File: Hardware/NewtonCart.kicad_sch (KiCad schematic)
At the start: 17 parts, among them J1 Battery Pins, J2 TP4056 Module, J3 Reserve IO's, J4 UART2TTL Bridge, J5 BoostConverter, J6 MPU6050, J7 HX711, J8 HC-SR04, J9 FOTOELECTRIC_ENCODER, U1 ESP32-WROOM-32, U2 LM1117-3.3

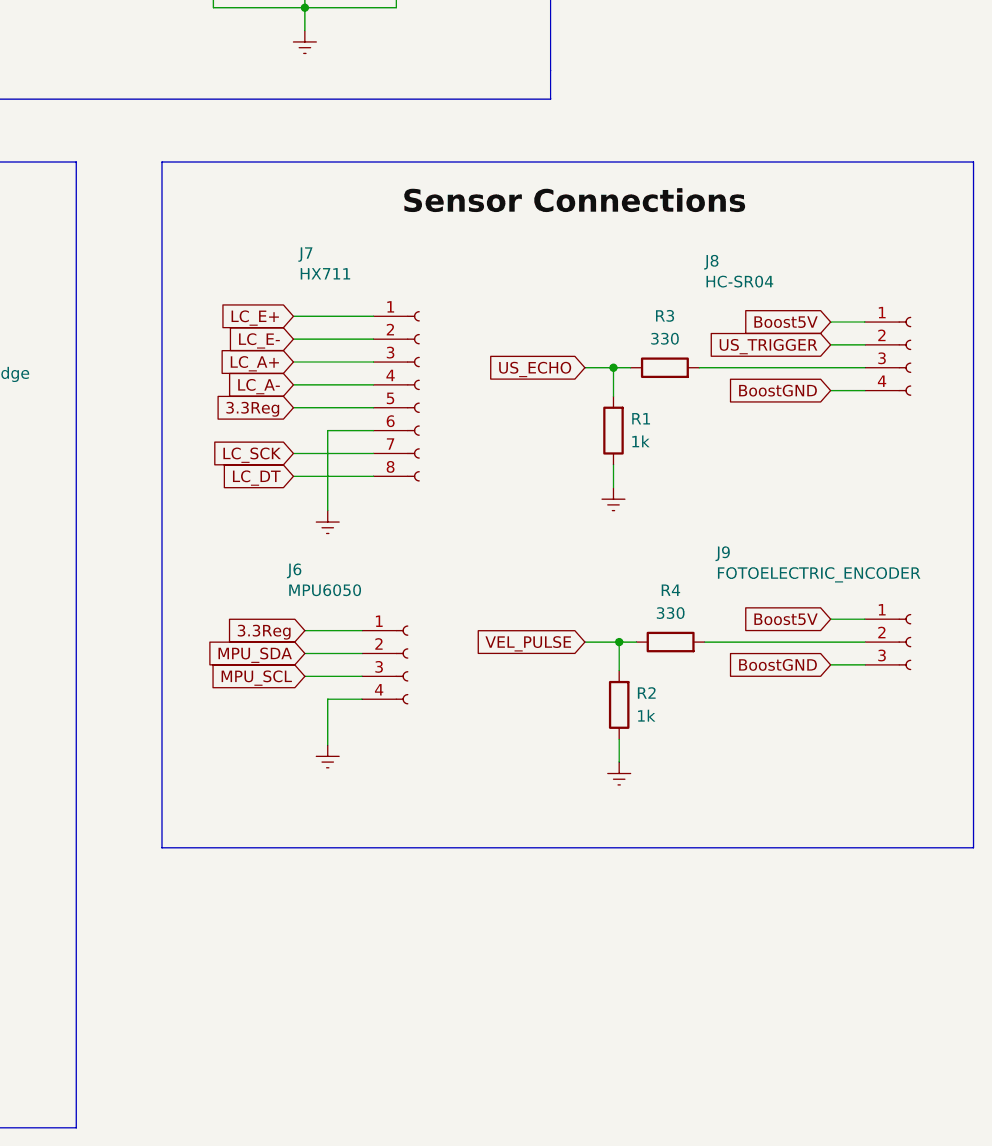
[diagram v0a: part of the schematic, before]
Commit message: Created Netlist, Locating PCB Boart components. Some schematic changes.
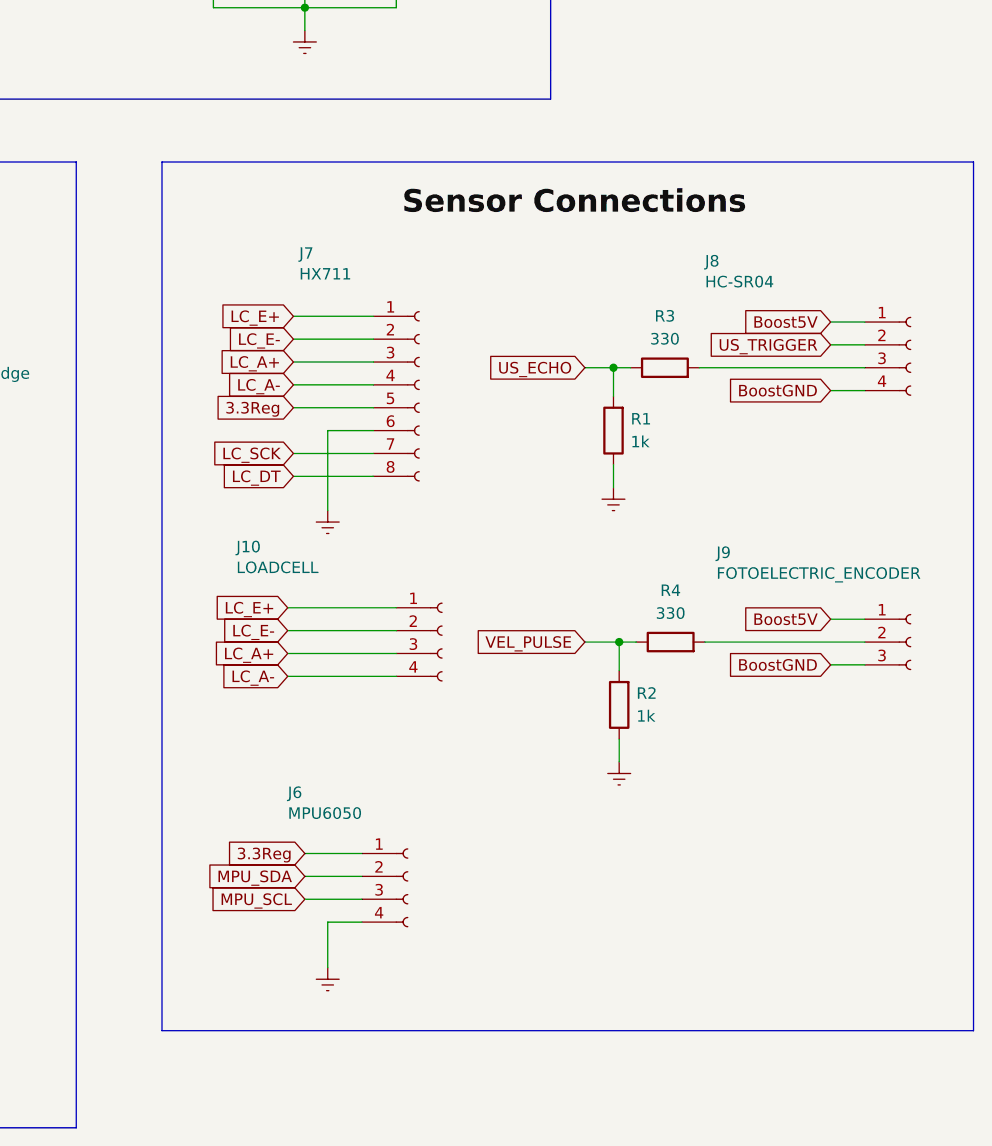
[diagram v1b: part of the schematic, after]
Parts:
- added J10: LOADCELL, Connector_PinHeader_2.54mm:PinHeader_1x04_P2.54mm_Vertical, symbol Connector:Conn_01x04_Female
- C1, C2: footprint (none) -> Resistor_THT:R_Axial_DIN0204_L3.6mm_D1.6mm_P5.08mm_Horizontal
- J1, J8: footprint (none) -> Connector_PinHeader_2.54mm:PinHeader_1x04_P2.54mm_Vertical
- J2: footprint (none) -> Miscelaneos:18650 TP4056 Module
- J3, J9: footprint (none) -> Connector_PinHeader_2.54mm:PinHeader_1x03_P2.54mm_Vertical
- J4: footprint (none) -> Connector_PinHeader_2.54mm:PinHeader_1x05_P2.54mm_Vertical
- J5: footprint (none) -> Miscelaneos:5-12V BoostConverter
- J6: footprint (none) -> Miscelaneos:MPU 6050 Module
- J7: footprint (none) -> Miscelaneos:HX711 Loadcell ADC
- R1, R2, R3, R4: footprint (none) -> Resistor_THT:R_Axial_DIN0309_L9.0mm_D3.2mm_P12.70mm_Horizontal
- U2: footprint (none) -> Package_TO_SOT_THT:TO-220-3_Vertical
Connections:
- net LC_A+: now also J10.3 (Pin_3)
- net LC_A-: now also J10.4 (Pin_4)
- net LC_E+: now also J10.1 (Pin_1)
- net LC_E-: now also J10.2 (Pin_2)
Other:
- moved on the sheet: J6

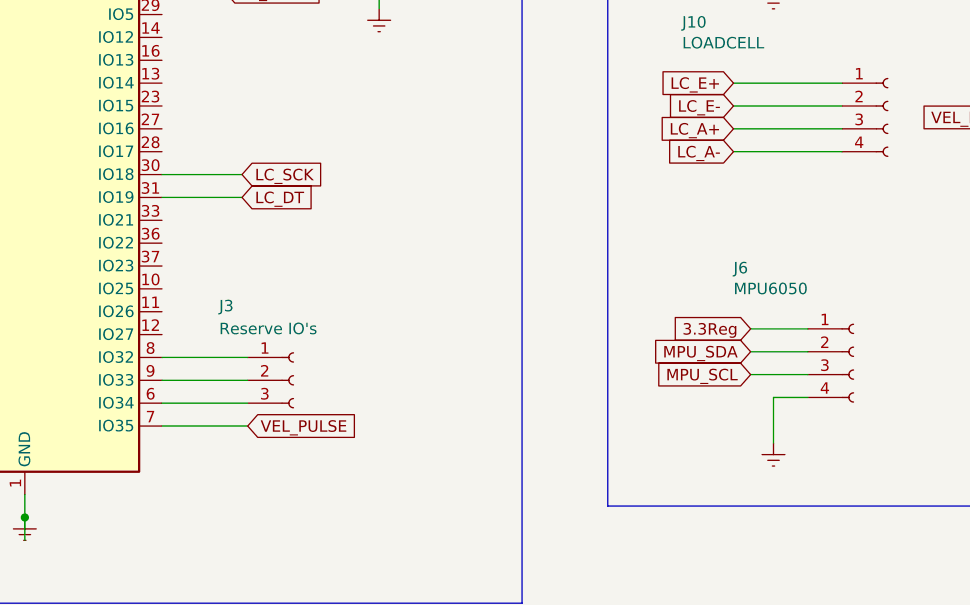
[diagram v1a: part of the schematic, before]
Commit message: Cambios Placa al 190322
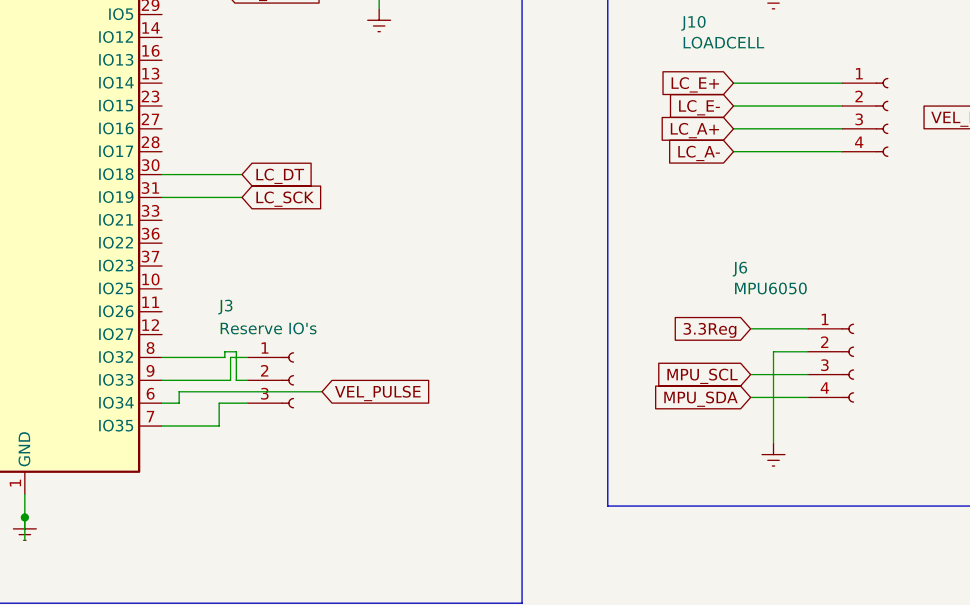
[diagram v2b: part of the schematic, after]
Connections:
- net Earth: now also J6.2 (Pin_2); no longer J6.4 (Pin_4)
- net LC_DT: now also U1.30 (IO18); no longer U1.31 (IO19)
- net LC_SCK: now also U1.31 (IO19); no longer U1.30 (IO18)
- net MPU_SDA: now also J6.4 (Pin_4); no longer J6.2 (Pin_2)
- net VEL_PULSE: now also U1.6 (IO34); no longer U1.7 (IO35)
- net at J3.3 (Pin_3): now also U1.7 (IO35); no longer U1.6 (IO34)
- net at U1.8 (IO32): now also J3.2 (Pin_2); no longer J3.1 (Pin_1)
- net at U1.9 (IO33): now also J3.1 (Pin_1); no longer J3.2 (Pin_2)
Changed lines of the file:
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@@
+    (stroke (width 0) (type default) (color 0 0 0 0))
+  )
+  (wire (pts (xy 145.415 147.955) (xy 151.765 147.955))
     (stroke (width 0) (type default) (color 0 0 0 0))
   )
@@
     (stroke (width 0) (type default) (color 0 0 0 0))
   )
+  (wire (pts (xy 147.955 145.415) (xy 147.955 155.575))
+    (stroke (width 0) (type default) (color 0 0 0 0))
+  )
   (wire (pts (xy 105.41 92.71) (xy 91.44 92.71))
     (stroke (width 0) (type default) (color 0 0 0 0))
   )
-  (wire (pts (xy 151.765 150.495) (xy 147.955 150.495))
-    (stroke (width 0) (type default) (color 0 0 0 0))
-  )
   (wire (pts (xy 203.835 116.84) (xy 207.645 116.84))
     (stroke (width 0) (type default) (color 0 0 0 0))
@@
     (stroke (width 0) (type default) (color 0 0 0 0))
   )
+  (wire (pts (xy 80.01 128.27) (xy 88.9 128.27))
+    (stroke (width 0) (type default) (color 0 0 0 0))
+  )
   (polyline (pts (xy 19.685 59.055) (xy 19.685 16.51))
     (stroke (width 0) (type default) (color 0 0 0 0))
@@
     (stroke (width 0) (type default) (color 0 0 0 0))
   )
-  (wire (pts (xy 80.01 148.59) (xy 89.535 148.59))
+  (wire (pts (xy 89.535 146.05) (xy 87.63 146.05))
+    (stroke (width 0) (type default) (color 0 0 0 0))
+  )
+  (wire (pts (xy 97.79 149.86) (xy 81.915 149.86))
     (stroke (width 0) (type default) (color 0 0 0 0))
   )
@@
     (stroke (width 0) (type default) (color 0 0 0 0))
   )
+  (wire (pts (xy 88.265 145.415) (xy 86.995 145.415))
+    (stroke (width 0) (type default) (color 0 0 0 0))
+  )
+  (wire (pts (xy 80.01 125.73) (xy 88.9 125.73))
+    (stroke (width 0) (type default) (color 0 0 0 0))
+  )
   (wire (pts (xy 101.6 100.33) (xy 101.6 102.87))
     (stroke (width 0) (type default) (color 0 0 0 0))
@@
     (stroke (width 0) (type default) (color 0 0 0 0))
   )
-  (wire (pts (xy 80.01 151.13) (xy 89.535 151.13))
+  (wire (pts (xy 81.915 151.13) (xy 80.01 151.13))
+    (stroke (width 0) (type default) (color 0 0 0 0))
+  )
+  (wire (pts (xy 87.63 148.59) (xy 80.01 148.59))
     (stroke (width 0) (type default) (color 0 0 0 0))
   )
@@
     (stroke (width 0) (type default) (color 0 0 0 0))
   )
-  (wire (pts (xy 80.01 125.73) (xy 88.9 125.73))
+  (wire (pts (xy 88.265 148.59) (xy 88.265 145.415))
     (stroke (width 0) (type default) (color 0 0 0 0))
   )
@@
     (stroke (width 0) (type default) (color 0 0 0 0))
   )
-  (wire (pts (xy 80.01 146.05) (xy 89.535 146.05))
-    (stroke (width 0) (type default) (color 0 0 0 0))
-  )
   (wire (pts (xy 73.66 41.275) (xy 77.47 41.275))
     (stroke (width 0) (type default) (color 0 0 0 0))
@@
     (stroke (width 0) (type default) (color 0 0 0 0))
   )
+  (wire (pts (xy 147.955 145.415) (xy 151.765 145.415))
+    (stroke (width 0) (type default) (color 0 0 0 0))
+  )
+  (wire (pts (xy 86.995 145.415) (xy 86.995 146.05))
+    (stroke (width 0) (type default) (color 0 0 0 0))
+  )
   (wire (pts (xy 91.44 80.645) (xy 94.615 80.645))
     (stroke (width 0) (type default) (color 0 0 0 0))
@@
     (stroke (width 0) (type default) (color 0 0 0 0))
   )
-  (wire (pts (xy 147.955 150.495) (xy 147.955 155.575))
-    (stroke (width 0) (type default) (color 0 0 0 0))
-  )
   (wire (pts (xy 35.56 46.99) (xy 39.37 46.99))
     (stroke (width 0) (type default) (color 0 0 0 0))
@@
     (stroke (width 0) (type default) (color 0 0 0 0))
   )
+  (wire (pts (xy 86.995 146.05) (xy 80.01 146.05))
+    (stroke (width 0) (type default) (color 0 0 0 0))
+  )
+  (wire (pts (xy 86.36 153.67) (xy 80.01 153.67))
+    (stroke (width 0) (type default) (color 0 0 0 0))
+  )
+  (wire (pts (xy 145.415 150.495) (xy 151.765 150.495))
+    (stroke (width 0) (type default) (color 0 0 0 0))
+  )
   (wire (pts (xy 143.51 120.65) (xy 155.575 120.65))
     (stroke (width 0) (type default) (color 0 0 0 0))
@@
     (stroke (width 0) (type default) (color 0 0 0 0))
   )
-  (wire (pts (xy 151.765 145.415) (xy 145.415 145.415))
-    (stroke (width 0) (type default) (color 0 0 0 0))
-  )
   (wire (pts (xy 203.835 83.82) (xy 207.645 83.82))
     (stroke (width 0) (type default) (color 0 0 0 0))
@@
     (stroke (width 0) (type default) (color 0 0 0 0))
   )
+  (wire (pts (xy 89.535 151.13) (xy 86.36 151.13))
+    (stroke (width 0) (type default) (color 0 0 0 0))
+  )
   (wire (pts (xy 129.54 37.465) (xy 135.255 37.465))
     (stroke (width 0) (type default) (color 0 0 0 0))
@@
     (stroke (width 0) (type default) (color 0 0 0 0))
   )
+  (wire (pts (xy 86.36 151.13) (xy 86.36 153.67))
+    (stroke (width 0) (type default) (color 0 0 0 0))
+  )
   (wire (pts (xy 203.835 121.92) (xy 207.645 121.92))
     (stroke (width 0) (type default) (color 0 0 0 0))
@@
     (stroke (width 0) (type default) (color 0 0 0 0))
   )
-  (wire (pts (xy 151.765 147.955) (xy 145.415 147.955))
-    (stroke (width 0) (type default) (color 0 0 0 0))
-  )
   (polyline (pts (xy 19.685 16.51) (xy 172.72 16.51))
     (stroke (width 0) (type default) (color 0 0 0 0))
   )
-  (wire (pts (xy 80.01 128.27) (xy 88.9 128.27))
+  (wire (pts (xy 81.915 149.86) (xy 81.915 151.13))
     (stroke (width 0) (type default) (color 0 0 0 0))
   )
@@
     (stroke (width 0) (type default) (color 0 0 0 0))
   )
+  (wire (pts (xy 89.535 148.59) (xy 88.265 148.59))
+    (stroke (width 0) (type default) (color 0 0 0 0))
+  )
   (wire (pts (xy 101.6 102.87) (xy 80.01 102.87))
     (stroke (width 0) (type default) (color 0 0 0 0))
@@
     (stroke (width 0) (type default) (color 0 0 0 0))
   )
+  (wire (pts (xy 87.63 146.05) (xy 87.63 148.59))
+    (stroke (width 0) (type default) (color 0 0 0 0))
+  )
   (wire (pts (xy 29.21 39.37) (xy 35.56 39.37))
-    (stroke (width 0) (type default) (color 0 0 0 0))
-  )
-  (wire (pts (xy 80.01 153.67) (xy 89.535 153.67))
     (stroke (width 0) (type default) (color 0 0 0 0))
   )
@@
     )
   )
-  (global_label "VEL_PULSE" (shape input) (at 89.535 153.67 0) (fields_autoplaced)
-    (effects (font (size 1.27 1.27)) (justify left))
-    (property "Intersheet References" "${INTERSHEET_REFS}" (id 0) (at 102.0797 153.5906 0)
+  (global_label "VEL_PULSE" (shape input) (at 97.79 149.86 0) (fields_autoplaced)
+    (effects (font (size 1.27 1.27)) (justify left))
+    (property "Intersheet References" "${INTERSHEET_REFS}" (id 0) (at 110.3347 149.7806 0)
       (effects (font (size 1.27 1.27)) (justify left) hide)
     )
@@
     )
   )
-  (global_label "LC_DT" (shape input) (at 88.9 128.27 0) (fields_autoplaced)
-    (effects (font (size 1.27 1.27)) (justify left))
-    (property "Intersheet References" "${INTERSHEET_REFS}" (id 0) (at -10.16 6.35 0)
+  (global_label "LC_DT" (shape input) (at 88.9 125.73 0) (fields_autoplaced)
+    (effects (font (size 1.27 1.27)) (justify left))
+    (property "Intersheet References" "${INTERSHEET_REFS}" (id 0) (at -10.16 3.81 0)
       (effects (font (size 1.27 1.27)) hide)
     )
@@
     )
   )
-  (global_label "LC_SCK" (shape input) (at 88.9 125.73 0) (fields_autoplaced)
-    (effects (font (size 1.27 1.27)) (justify left))
-    (property "Intersheet References" "${INTERSHEET_REFS}" (id 0) (at -10.16 7.62 0)
-      (effects (font (size 1.27 1.27)) hide)
-    )
-  )
-  (global_label "MPU_SDA" (shape input) (at 145.415 145.415 180) (fields_autoplaced)
-    (effects (font (size 1.27 1.27)) (justify right))
-    (property "Intersheet References" "${INTERSHEET_REFS}" (id 0) (at 12.065 38.735 0)
-      (effects (font (size 1.27 1.27)) hide)
-    )
+  (global_label "LC_SCK" (shape input) (at 88.9 128.27 0) (fields_autoplaced)
+    (effects (font (size 1.27 1.27)) (justify left))
+    (property "Intersheet References" "${INTERSHEET_REFS}" (id 0) (at -10.16 10.16 0)
+      (effects (font (size 1.27 1.27)) hide)
+    )
+  )
+  (global_label "MPU_SDA" (shape input) (at 145.415 150.495 180) (fields_autoplaced)
+    (effects (font (size 1.27 1.27)) (justify right))
+    (property "Intersheet References" "${INTERSHEET_REFS}" (id 0) (at 12.065 43.815 0)
+      (effects (font (size 1.27 1.27)) hide)
+    )
